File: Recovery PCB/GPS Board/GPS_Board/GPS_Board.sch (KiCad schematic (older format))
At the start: 10 parts

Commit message: more recovery pcb shid
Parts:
- added TP?: TestPoint, TestPoint:TestPoint_Pad_D1.0mm, symbol Connector:TestPoint
- A: footprint (none) -> GPS Board:XBEE-20_THT
- A?: footprint (none) -> GPS Board:EBOOT-MP1584EN-5N-POWER-SUPPLY
- J? (x2): footprint (none) -> Connector_AMASS:AMASS_XT30U-M_1x02_P5.0mm_Vertical
- TP? (x4): footprint (none) -> TestPoint:TestPoint_Pad_D1.5mm
- U?: footprint (none) -> teensy:Teensy41
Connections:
- wire segments 35 -> 77
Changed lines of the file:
@@
 F 0 "U?" H 2900 6115 50  0000 C CNN
 F 1 "Teensy4.1" H 2900 6024 50  0000 C CNN
-F 2 "" H 2500 3950 50  0001 C CNN
+F 2 "teensy:Teensy41" H 2500 3950 50  0001 C CNN
 F 3 "" H 2500 3950 50  0001 C CNN
 	1    2900 3550
@@
 F 0 "A?" H 9400 2615 50  0000 C CNN
 F 1 "Eboot-MP1584EN-5V-Power-Supply" H 9400 2524 50  0000 C CNN
-F 2 "" H 9400 1950 50  0001 C CNN
+F 2 "GPS Board:EBOOT-MP1584EN-5N-POWER-SUPPLY" H 9400 1950 50  0001 C CNN
 F 3 "" H 9400 1950 50  0001 C CNN
 	1    9400 1950
@@
 F 0 "J?" V 7216 2468 50  0000 L CNN
 F 1 "XT30-M" V 7307 2468 50  0000 L CNN
-F 2 "" H 7250 2000 50  0001 C CNN
+F 2 "Connector_AMASS:AMASS_XT30U-M_1x02_P5.0mm_Vertical" H 7250 2000 50  0001 C CNN
 F 3 "" H 7250 2000 50  0001 C CNN
 	1    7250 2000
@@
 F 0 "J?" H 7923 2466 50  0000 R CNN
 F 1 "XT30-M" H 7923 2557 50  0000 R CNN
-F 2 "" H 8100 2300 50  0001 C CNN
+F 2 "Connector_AMASS:AMASS_XT30U-M_1x02_P5.0mm_Vertical" H 8100 2300 50  0001 C CNN
 F 3 "" H 8100 2300 50  0001 C CNN
 	1    8100 2300
@@
 F 0 "A" H 5825 2665 50  0000 C CNN
 F 1 "XBee-3-Pro" H 5825 2574 50  0000 C CNN
-F 2 "" H 5825 1900 50  0001 C CNN
+F 2 "GPS Board:XBEE-20_THT" H 5825 1900 50  0001 C CNN
 F 3 "" H 5825 1900 50  0001 C CNN
 	1    5825 1900
@@
 F 0 "TP?" V 5745 3522 50  0000 C CNN
 F 1 "TestPoint" V 5654 3522 50  0000 C CNN
-F 2 "" H 5750 3450 50  0001 C CNN
+F 2 "TestPoint:TestPoint_Pad_D1.5mm" H 5750 3450 50  0001 C CNN
 F 3 "~" H 5750 3450 50  0001 C CNN
 	1    5550 3450
@@
 F 0 "TP?" V 5745 3597 50  0000 C CNN
 F 1 "TestPoint" V 5654 3597 50  0000 C CNN
-F 2 "" H 5750 3525 50  0001 C CNN
+F 2 "TestPoint:TestPoint_Pad_D1.5mm" H 5750 3525 50  0001 C CNN
 F 3 "~" H 5750 3525 50  0001 C CNN
 	1    5550 3525
@@
 F 0 "TP?" H 2842 4876 50  0000 R CNN
 F 1 "TestPoint" H 2842 4967 50  0000 R CNN
-F 2 "" H 3100 4850 50  0001 C CNN
+F 2 "TestPoint:TestPoint_Pad_D1.5mm" H 3100 4850 50  0001 C CNN
 F 3 "~" H 3100 4850 50  0001 C CNN
 	1    2900 4850
@@
 F 0 "TP?" H 2542 4876 50  0000 R CNN
 F 1 "TestPoint" H 2542 4967 50  0000 R CNN
-F 2 "" H 2800 4850 50  0001 C CNN
+F 2 "TestPoint:TestPoint_Pad_D1.5mm" H 2800 4850 50  0001 C CNN
 F 3 "~" H 2800 4850 50  0001 C CNN
 	1    2600 4850
@@
 	1    0    0    -1
 $EndComp
+Wire Wire Line
+	5500 1425 4350 1425
+Wire Wire Line
+	4350 1425 4350 1600
+Connection ~ 4350 1600
+$Comp
+L Connector:TestPoint TP?
+U 1 1 61AB1BEF
+P 6150 1475
+F 0 "TP?" V 6104 1663 50  0000 L CNN
+F 1 "TestPoint" V 6195 1663 50  0000 L CNN
+F 2 "TestPoint:TestPoint_Pad_D1.0mm" H 6350 1475 50  0001 C CNN
+F 3 "~" H 6350 1475 50  0001 C CNN
+	1    6150 1475
+	0    1    1    0
+$EndComp
+Wire Wire Line
+	5500 1575 5300 1575
+Wire Wire Line
+	5300 1575 5300 750
+Wire Wire Line
+	5300 750  1250 750
+Wire Wire Line
+	1250 750  1250 2700
+Wire Wire Line
+	1250 2700 1800 2700
+Wire Wire Line
+	5500 1675 4175 1675
+Wire Wire Line
+	4175 1675 4175 1800
+Wire Wire Line
+	4175 1800 4000 1800
+Wire Wire Line
+	5500 1625 4775 1625
+Wire Wire Line
+	4775 1625 4775 3300
+Wire Wire Line
+	4775 3300 4000 3300
+Wire Wire Line
+	6425 3550 6625 3550
+Wire Wire Line
+	6625 3550 6625 4275
+Wire Wire Line
+	6625 4275 4750 4275
+Wire Wire Line
+	4750 4275 4750 3400
+Wire Wire Line
+	4750 3400 4000 3400
+Wire Wire Line
+	5500 1825 5375 1825
+Wire Wire Line
+	5375 1825 5375 3200
+Wire Wire Line
+	5375 3200 4000 3200
+Wire Wire Line
+	6150 1875 6650 1875
+Wire Wire Line
+	6650 1875 6650 850
+Wire Wire Line
+	6650 850  1375 850
+Wire Wire Line
+	1375 850  1375 2600
+Wire Wire Line
+	1375 2600 1800 2600
+Wire Wire Line
+	1800 2500 1475 2500
+Wire Wire Line
+	1475 2500 1475 950
+Wire Wire Line
+	1475 950  6500 950
+Wire Wire Line
+	6500 950  6500 1575
+Wire Wire Line
+	6500 1575 6150 1575
+Wire Wire Line
+	6150 1525 6425 1525
+Wire Wire Line
+	6425 1525 6425 1075
+Wire Wire Line
+	6425 1075 4550 1075
+Wire Wire Line
+	4550 1075 4550 2700
+Wire Wire Line
+	4550 2700 4000 2700
+Wire Wire Line
+	6150 1775 6150 1825
+Wire Wire Line
+	6150 2925 4525 2925
+Wire Wire Line
+	4525 2925 4525 3700
+Wire Wire Line
+	4525 3700 4000 3700
+Connection ~ 6150 1825
+Wire Wire Line
+	6150 1825 6150 1875
+Connection ~ 6150 1875
+Wire Wire Line
+	6150 1875 6150 2925
 $EndSCHEMATC

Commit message: recovery board changes
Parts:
- U1: renamed from U?; footprint teensy:Teensy41 -> GPS Board:Teensy41; symbol teensy:Teensy4.1 -> GPS_Board-rescue:Teensy4.1-teensy
- gave numbers to parts that had none: 9
- renumbered A to A1
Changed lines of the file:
@@
 $EndDescr
 $Comp
-L teensy:Teensy4.1 U?
+L GPS_Board-rescue:Teensy4.1-teensy U1
 U 1 1 61A899BD
 P 2900 3550
-F 0 "U?" H 2900 6115 50  0000 C CNN
+F 0 "U1" H 2900 6115 50  0000 C CNN
 F 1 "Teensy4.1" H 2900 6024 50  0000 C CNN
-F 2 "teensy:Teensy41" H 2500 3950 50  0001 C CNN
+F 2 "GPS Board:Teensy41" H 2500 3950 50  0001 C CNN
 F 3 "" H 2500 3950 50  0001 C CNN
 	1    2900 3550
@@
 $EndComp
 $Comp
-L eboot-mp1584en-5v-power-supply:Eboot-MP1584EN-5V-Power-Supply A?
+L eboot-mp1584en-5v-power-supply:Eboot-MP1584EN-5V-Power-Supply A3
 U 1 1 61A8FD6D
 P 9400 1950
-F 0 "A?" H 9400 2615 50  0000 C CNN
+F 0 "A3" H 9400 2615 50  0000 C CNN
 F 1 "Eboot-MP1584EN-5V-Power-Supply" H 9400 2524 50  0000 C CNN
 F 2 "GPS Board:EBOOT-MP1584EN-5N-POWER-SUPPLY" H 9400 1950 50  0001 C CNN
@@
 $EndComp
 $Comp
-L GPS_Board:XT30-M J?
+L GPS_Board:XT30-M J1
 U 1 1 61A95F1A
 P 7250 2000
-F 0 "J?" V 7216 2468 50  0000 L CNN
+F 0 "J1" V 7216 2468 50  0000 L CNN
 F 1 "XT30-M" V 7307 2468 50  0000 L CNN
 F 2 "Connector_AMASS:AMASS_XT30U-M_1x02_P5.0mm_Vertical" H 7250 2000 50  0001 C CNN
@@
 $EndComp
 $Comp
-L GPS_Board:XT30-M J?
+L GPS_Board:XT30-M J2
 U 1 1 61A98361
 P 8100 2300
-F 0 "J?" H 7923 2466 50  0000 R CNN
+F 0 "J2" H 7923 2466 50  0000 R CNN
 F 1 "XT30-M" H 7923 2557 50  0000 R CNN
 F 2 "Connector_AMASS:AMASS_XT30U-M_1x02_P5.0mm_Vertical" H 8100 2300 50  0001 C CNN
@@
 	7075 1925 7250 1925
 $Comp
-L GPS_Board:Sparkfun-GPS-Breakout A?
+L GPS_Board:Sparkfun-GPS-Breakout A2
 U 1 1 61AAF79D
 P 6000 3900
-F 0 "A?" H 6050 4640 50  0000 C CNN
+F 0 "A2" H 6050 4640 50  0000 C CNN
 F 1 "Sparkfun-GPS-Breakout" H 6050 4549 50  0000 C CNN
 F 2 "" H 6000 3900 50  0001 C CNN
@@
 $EndComp
 $Comp
-L GPS_Board:XBee-3-Pro A
+L GPS_Board:XBee-3-Pro A1
 U 1 1 61AB64FA
 P 5825 1900
-F 0 "A" H 5825 2665 50  0000 C CNN
+F 0 "A1" H 5825 2665 50  0000 C CNN
 F 1 "XBee-3-Pro" H 5825 2574 50  0000 C CNN
 F 2 "GPS Board:XBEE-20_THT" H 5825 1900 50  0001 C CNN
@@
 $EndComp
 $Comp
-L Connector:TestPoint TP?
+L Connector:TestPoint TP3
 U 1 1 61AB8223
 P 5550 3450
-F 0 "TP?" V 5745 3522 50  0000 C CNN
+F 0 "TP3" V 5745 3522 50  0000 C CNN
 F 1 "TestPoint" V 5654 3522 50  0000 C CNN
 F 2 "TestPoint:TestPoint_Pad_D1.5mm" H 5750 3450 50  0001 C CNN
@@
 $EndComp
 $Comp
-L Connector:TestPoint TP?
+L Connector:TestPoint TP4
 U 1 1 61AB9396
 P 5550 3525
-F 0 "TP?" V 5745 3597 50  0000 C CNN
+F 0 "TP4" V 5745 3597 50  0000 C CNN
 F 1 "TestPoint" V 5654 3597 50  0000 C CNN
 F 2 "TestPoint:TestPoint_Pad_D1.5mm" H 5750 3525 50  0001 C CNN
@@
 	5175 3750 5675 3750
 $Comp
-L power:GND #PWR?
+L power:GND #PWR0101
 U 1 1 61ABCD1D
 P 5675 3650
-F 0 "#PWR?" H 5675 3400 50  0001 C CNN
+F 0 "#PWR0101" H 5675 3400 50  0001 C CNN
 F 1 "GND" V 5680 3522 50  0000 R CNN
 F 2 "" H 5675 3650 50  0001 C CNN
@@
 	4350 1600 4000 1600
 $Comp
-L power:GND #PWR?
+L power:GND #PWR0102
 U 1 1 61ABF5FF
 P 1800 1400
-F 0 "#PWR?" H 1800 1150 50  0001 C CNN
+F 0 "#PWR0102" H 1800 1150 50  0001 C CNN
 F 1 "GND" V 1805 1272 50  0000 R CNN
 F 2 "" H 1800 1400 50  0001 C CNN
@@
 $EndComp
 $Comp
-L power:GND #PWR?
+L power:GND #PWR0103
 U 1 1 61AC06CC
 P 4000 1500
-F 0 "#PWR?" H 4000 1250 50  0001 C CNN
+F 0 "#PWR0103" H 4000 1250 50  0001 C CNN
 F 1 "GND" V 4005 1372 50  0000 R CNN
 F 2 "" H 4000 1500 50  0001 C CNN
@@
 $EndComp
 $Comp
-L power:GND #PWR?
+L power:GND #PWR0104
 U 1 1 61AC16D1
 P 10200 1550
-F 0 "#PWR?" H 10200 1300 50  0001 C CNN
+F 0 "#PWR0104" H 10200 1300 50  0001 C CNN
 F 1 "GND" V 10205 1422 50  0000 R CNN
 F 2 "" H 10200 1550 50  0001 C CNN
@@
 $EndComp
 $Comp
-L power:GND #PWR?
+L power:GND #PWR0105
 U 1 1 61AC2FBA
 P 4000 2800
-F 0 "#PWR?" H 4000 2550 50  0001 C CNN
+F 0 "#PWR0105" H 4000 2550 50  0001 C CNN
 F 1 "GND" V 4005 2672 50  0000 R CNN
 F 2 "" H 4000 2800 50  0001 C CNN
@@
 $EndComp
 $Comp
-L power:GND #PWR?
+L power:GND #PWR0106
 U 1 1 61ACAD1F
 P 5500 1875
-F 0 "#PWR?" H 5500 1625 50  0001 C CNN
+F 0 "#PWR0106" H 5500 1625 50  0001 C CNN
 F 1 "GND" H 5505 1702 50  0000 C CNN
 F 2 "" H 5500 1875 50  0001 C CNN
@@
 $EndComp
 $Comp
-L Connector:TestPoint TP?
+L Connector:TestPoint TP2
 U 1 1 61ACEA37
 P 2900 4850
-F 0 "TP?" H 2842 4876 50  0000 R CNN
+F 0 "TP2" H 2842 4876 50  0000 R CNN
 F 1 "TestPoint" H 2842 4967 50  0000 R CNN
 F 2 "TestPoint:TestPoint_Pad_D1.5mm" H 3100 4850 50  0001 C CNN
@@
 $EndComp
 $Comp
-L Connector:TestPoint TP?
+L Connector:TestPoint TP1
 U 1 1 61ACF9DD
 P 2600 4850
-F 0 "TP?" H 2542 4876 50  0000 R CNN
+F 0 "TP1" H 2542 4876 50  0000 R CNN
 F 1 "TestPoint" H 2542 4967 50  0000 R CNN
 F 2 "TestPoint:TestPoint_Pad_D1.5mm" H 2800 4850 50  0001 C CNN
@@
 $EndComp
 $Comp
-L power:+5V #PWR?
+L power:+5V #PWR0107
 U 1 1 61AD1665
 P 4000 1400
-F 0 "#PWR?" H 4000 1250 50  0001 C CNN
+F 0 "#PWR0107" H 4000 1250 50  0001 C CNN
 F 1 "+5V" V 4015 1528 50  0000 L CNN
 F 2 "" H 4000 1400 50  0001 C CNN
@@
 $EndComp
 $Comp
-L power:+5V #PWR?
+L power:+5V #PWR0108
 U 1 1 61AD2A6D
 P 10200 2400
-F 0 "#PWR?" H 10200 2250 50  0001 C CNN
+F 0 "#PWR0108" H 10200 2250 50  0001 C CNN
 F 1 "+5V" V 10215 2528 50  0000 L CNN
 F 2 "" H 10200 2400 50  0001 C CNN
@@
 Connection ~ 2900 4850
 $Comp
-L power:GND #PWR?
+L power:GND #PWR0109
 U 1 1 61ADB104
 P 2950 5125
-F 0 "#PWR?" H 2950 4875 50  0001 C CNN
+F 0 "#PWR0109" H 2950 4875 50  0001 C CNN
 F 1 "GND" H 2955 4952 50  0000 C CNN
 F 2 "" H 2950 5125 50  0001 C CNN
@@
 Connection ~ 4350 1600
 $Comp
-L Connector:TestPoint TP?
+L Connector:TestPoint TP5
 U 1 1 61AB1BEF
 P 6150 1475
-F 0 "TP?" V 6104 1663 50  0000 L CNN
+F 0 "TP5" V 6104 1663 50  0000 L CNN
 F 1 "TestPoint" V 6195 1663 50  0000 L CNN
 F 2 "TestPoint:TestPoint_Pad_D1.0mm" H 6350 1475 50  0001 C CNN

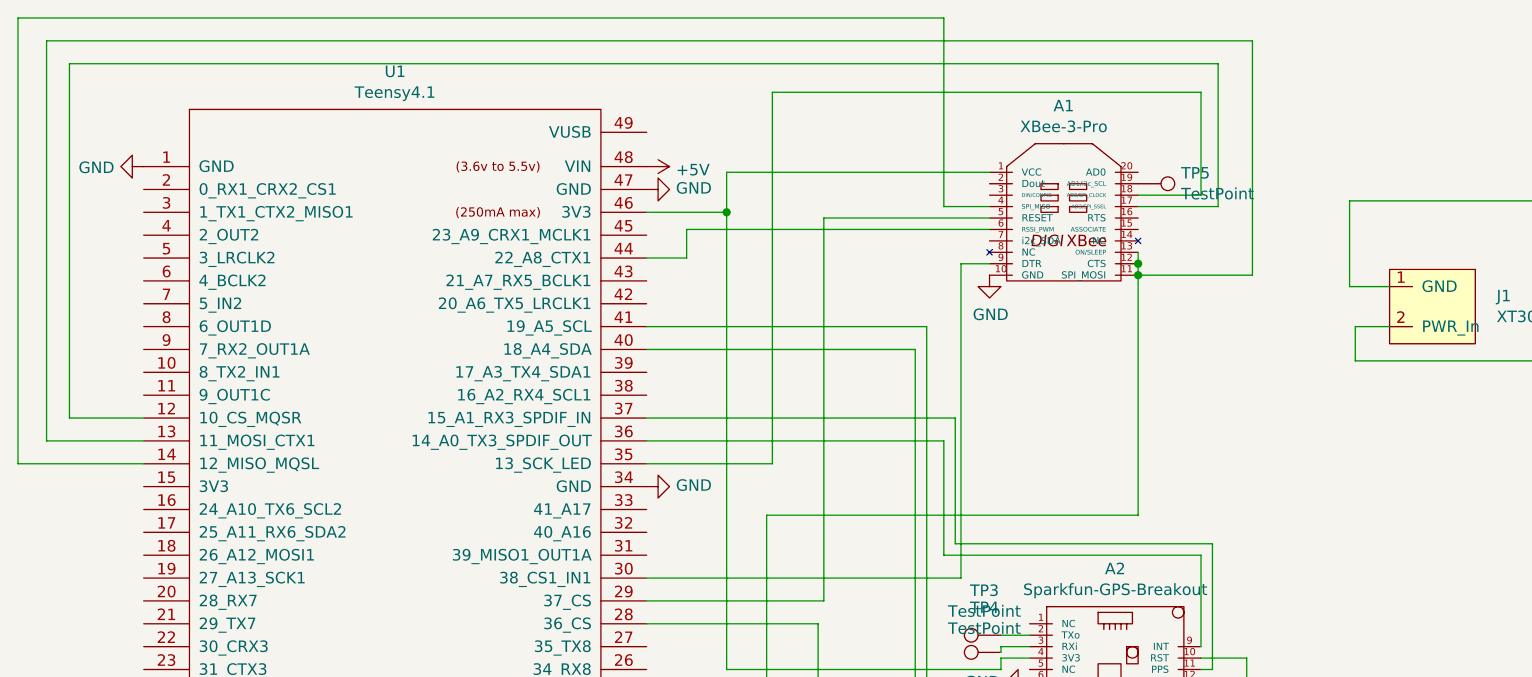
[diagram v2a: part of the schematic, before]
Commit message: finally opened my laptop and pushing changes and gerbers i sent to JLC
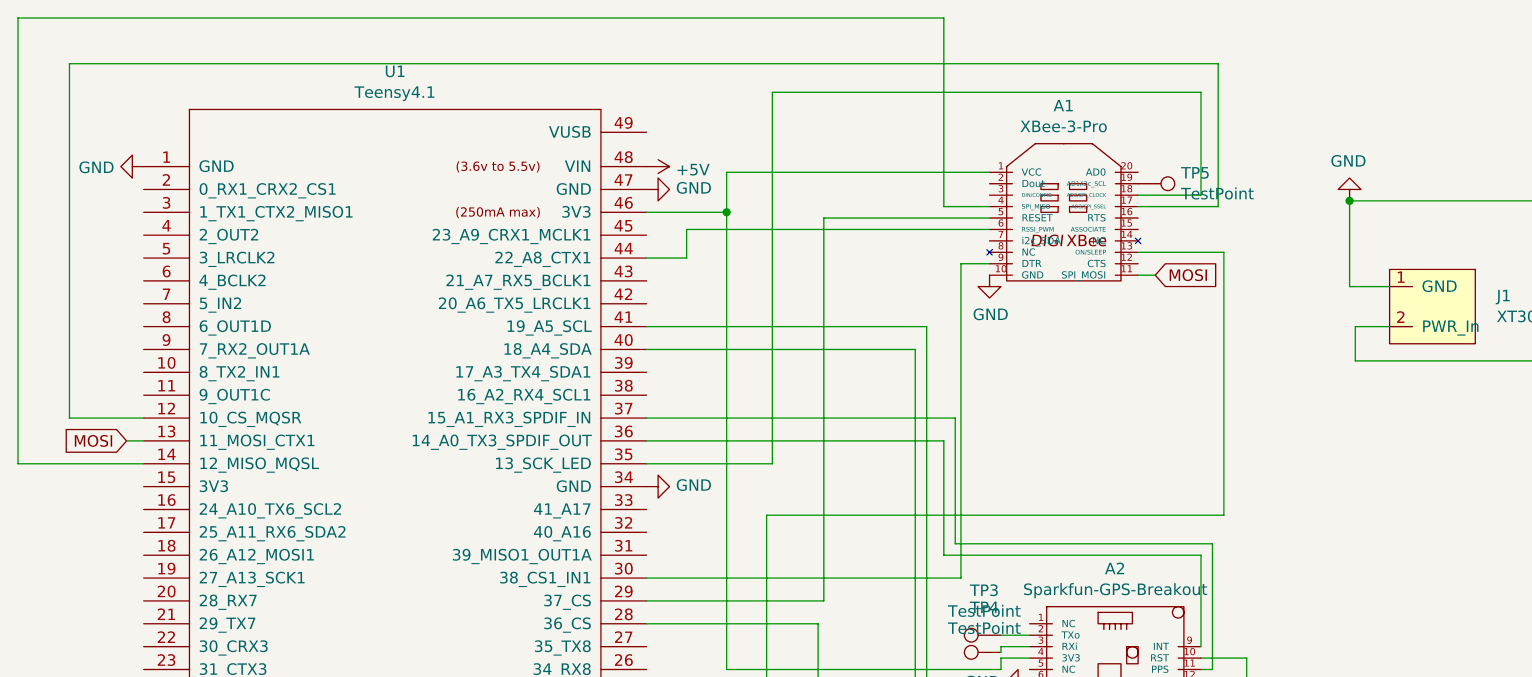
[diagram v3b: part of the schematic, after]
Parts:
- A2: footprint (none) -> GPS Board:Sparkfun-GPS-ZOE-M8Q-Breakout
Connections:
- net GND: now also A3.1 (GND_IN), J1.1 (GND)
- new net: A1.13 (ON/SLEEP), U1.25 (33_MCLK2)
- new net MOSI: A1.11 (SPI_MOSI), U1.13 (11_MOSI_CTX1)
- now unconnected: A1.12 (CTS)
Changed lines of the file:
@@
 F 0 "A2" H 6050 4640 50  0000 C CNN
 F 1 "Sparkfun-GPS-Breakout" H 6050 4549 50  0000 C CNN
-F 2 "" H 6000 3900 50  0001 C CNN
+F 2 "GPS Board:Sparkfun-GPS-ZOE-M8Q-Breakout" H 6000 3900 50  0001 C CNN
 F 3 "" H 6000 3900 50  0001 C CNN
 	1    6000 3900
@@
 	5375 3200 4000 3200
 Wire Wire Line
-	6150 1875 6650 1875
-Wire Wire Line
-	6650 1875 6650 850
-Wire Wire Line
-	6650 850  1375 850
-Wire Wire Line
-	1375 850  1375 2600
-Wire Wire Line
-	1375 2600 1800 2600
-Wire Wire Line
 	1800 2500 1475 2500
 Wire Wire Line
@@
 	4550 2700 4000 2700
 Wire Wire Line
-	6150 1775 6150 1825
-Wire Wire Line
-	6150 2925 4525 2925
-Wire Wire Line
 	4525 2925 4525 3700
 Wire Wire Line
 	4525 3700 4000 3700
-Connection ~ 6150 1825
-Wire Wire Line
-	6150 1825 6150 1875
-Connection ~ 6150 1875
-Wire Wire Line
-	6150 1875 6150 2925
+Text GLabel 6225 1875 2    50   Input ~ 0
+MOSI
+Wire Wire Line
+	6150 1875 6225 1875
+Wire Wire Line
+	6150 1775 6525 1775
+Wire Wire Line
+	4525 2925 6525 2925
+Wire Wire Line
+	6525 1775 6525 2925
+Text GLabel 1725 2600 0    50   Input ~ 0
+MOSI
+Wire Wire Line
+	1800 2600 1725 2600
+$Comp
+L power:GND #PWR?
+U 1 1 61BA5EBA
+P 7075 1550
+F 0 "#PWR?" H 7075 1300 50  0001 C CNN
+F 1 "GND" H 7080 1377 50  0000 C CNN
+F 2 "" H 7075 1550 50  0001 C CNN
+F 3 "" H 7075 1550 50  0001 C CNN
+	1    7075 1550
+	-1   0    0    1
+$EndComp
+Connection ~ 7075 1550
 $EndSCHEMATC
